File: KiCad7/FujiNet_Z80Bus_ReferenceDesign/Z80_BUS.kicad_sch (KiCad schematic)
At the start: 5 parts, among them J7 HOST SYSTEM HEADER, J8 DIAG-HOST_SYSTEM_BUS

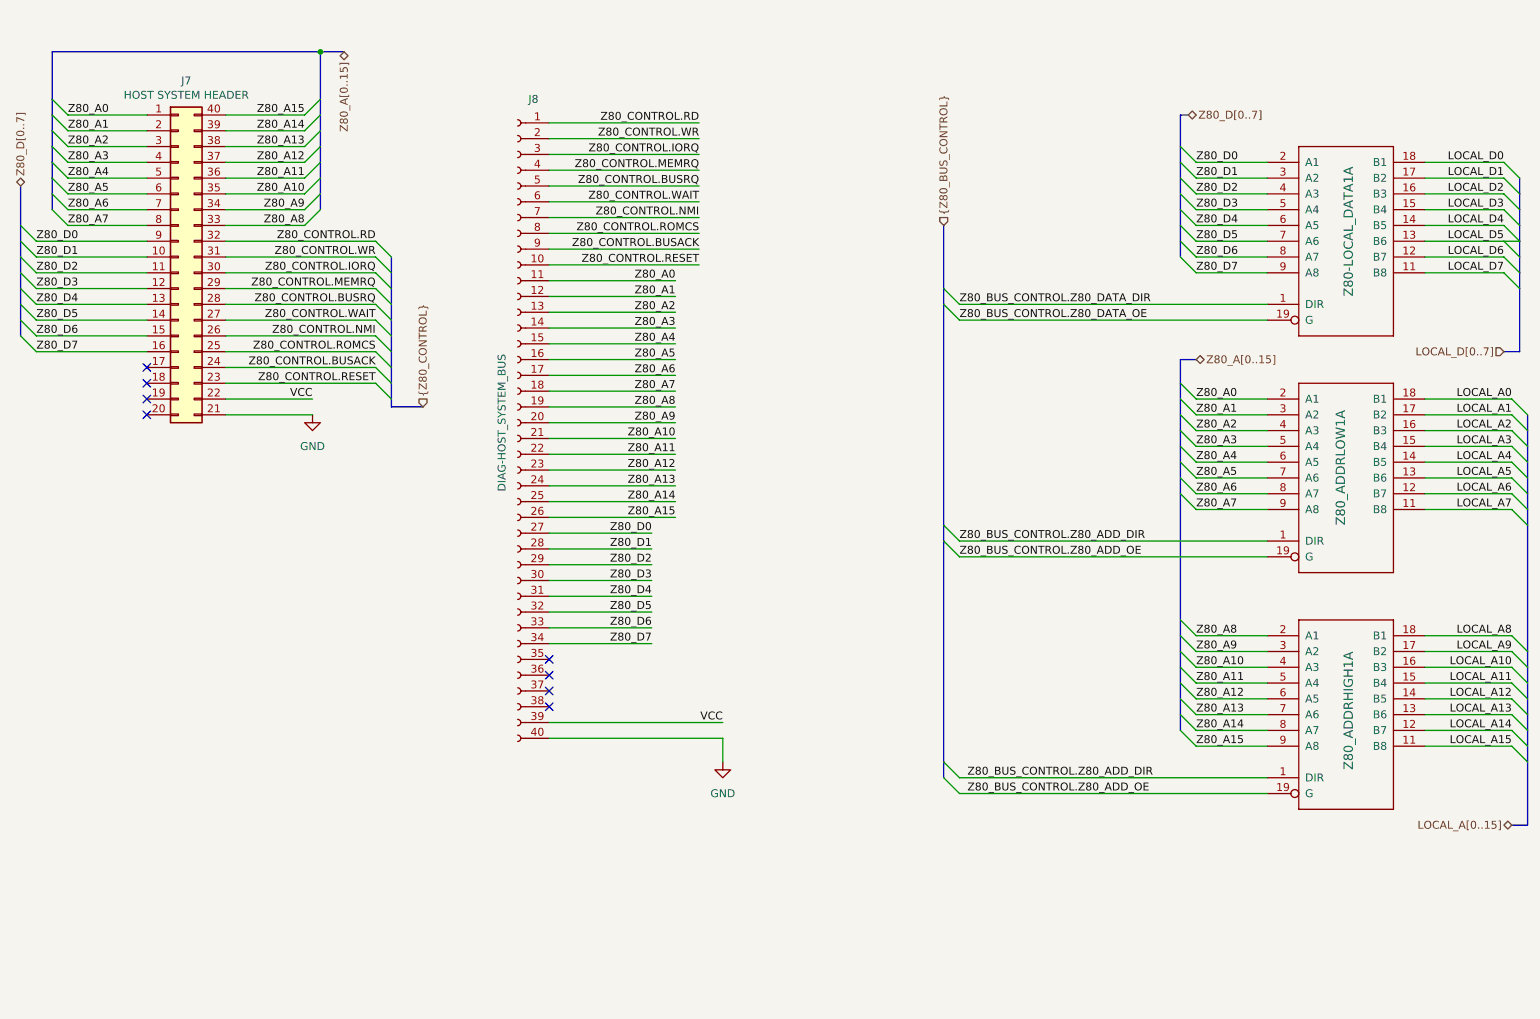
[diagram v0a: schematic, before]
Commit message: KiCad - ALMOST ERROR FREE!!!!
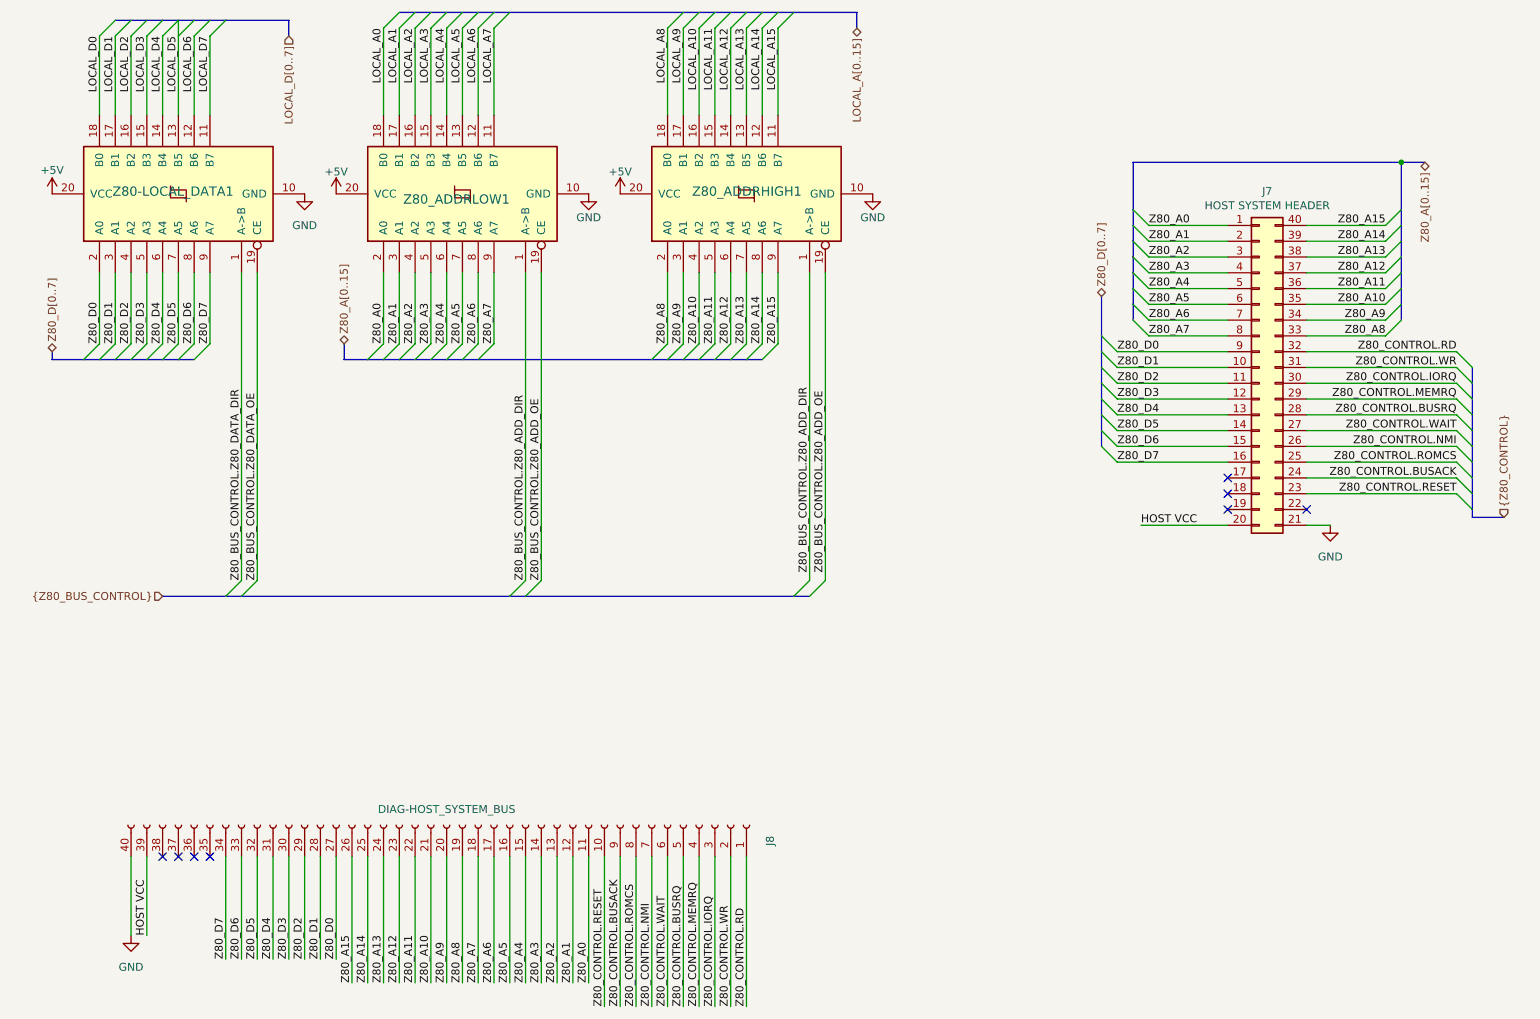
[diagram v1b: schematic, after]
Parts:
- Z80-LOCAL_DATA1, Z80_ADDRHIGH1, Z80_ADDRLOW1: symbol FujiNet_Z80Bus_Reference-rescue:74245N-Z80Decoder-eagle-import -> 74xx:74HC245
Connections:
- net GND: now also Z80-LOCAL_DATA1.10 (GND), Z80_ADDRHIGH1.10 (GND), Z80_ADDRLOW1.10 (GND)
- net HOST VCC: now reaches J7.20 (Pin_20)
- net HOST VCC: now also J8.39 (Pin_39)
- net VCC: no longer names the net of J7.22 (Pin_22)
- net VCC: no longer J8.39 (Pin_39)
- new net +5V: Z80-LOCAL_DATA1.20 (VCC), Z80_ADDRHIGH1.20 (VCC), Z80_ADDRLOW1.20 (VCC)
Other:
- moved on the sheet: J7, J8

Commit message: KiCAD PCB layout testing
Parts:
- Z80-LOCAL_DATA1, Z80_ADDRHIGH1, Z80_ADDRLOW1: value 74245N -> 74HC245N
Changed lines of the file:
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@@
       (effects (font (size 1.4986 1.4986)) (justify left bottom))
     )
-    (property "Value" "74245N" (at 74.93 53.34 0)
+    (property "Value" "74HC245N" (at 74.93 53.34 0)
       (effects (font (size 1.4986 1.4986)) (justify left bottom) hide)
     )
@@
       (effects (font (size 1.4986 1.4986)) (justify left bottom))
     )
-    (property "Value" "74245N" (at 166.37 53.34 0)
+    (property "Value" "74HC245N" (at 166.37 53.34 0)
       (effects (font (size 1.4986 1.4986)) (justify left bottom) hide)
     )
@@
       (effects (font (size 1.4986 1.4986)) (justify left bottom))
     )
-    (property "Value" "74245N" (at 120.65 53.34 0)
+    (property "Value" "74HC245N" (at 120.65 53.34 0)
       (effects (font (size 1.4986 1.4986)) (justify left bottom) hide)
     )
